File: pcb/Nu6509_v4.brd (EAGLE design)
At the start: 67.9 x 20.3 mm, 22 parts, among them IC1 6509, IC3 (C)02/'816, IC4 XC9572XL

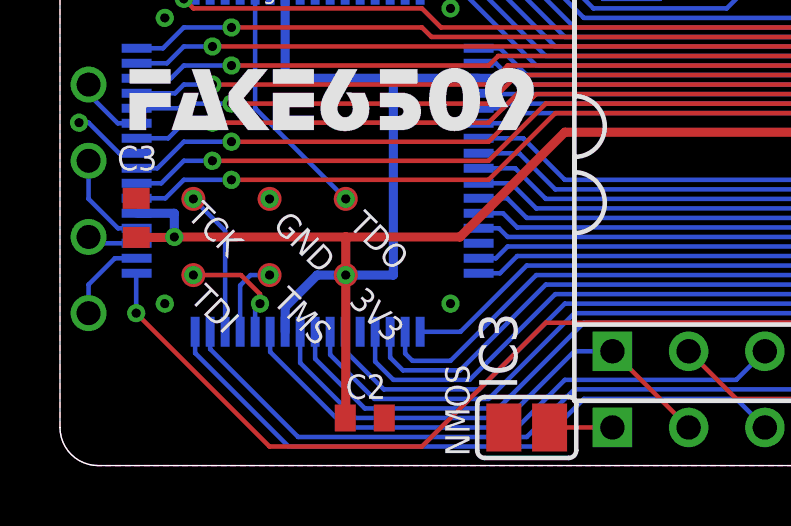
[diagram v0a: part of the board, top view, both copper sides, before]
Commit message: Switch name to Nu6509
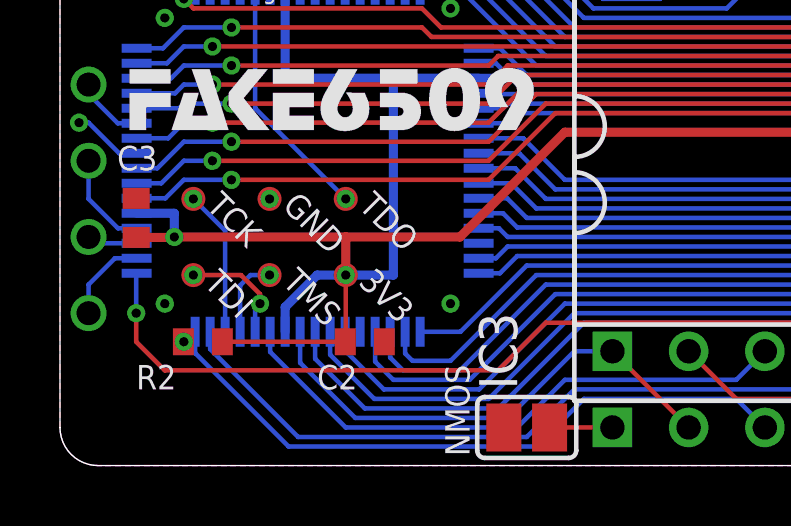
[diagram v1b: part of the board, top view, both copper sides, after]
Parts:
- added R2: 10K, rcl:R0402
- moved C2 2.54 mm to (-24.8, -6.03)
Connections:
- net !ABORT: now also R2.2
- net +3V3: now also R2.1
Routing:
- net +3V3: track 88.4 -> 90.0 mm
- net BE: track 96.6 -> 95.1 mm
- net !ABORT: track 22.0 -> 22.6 mm, vias 0 -> 1
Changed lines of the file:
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@@
 </autorouter>
 <elements>
-<element name="C2" library="rcl" package="C0402" value=".1" x="-24.765" y="-8.5725" smashed="yes">
-<attribute name="NAME" x="-25.4" y="-7.9375" size="0.8128" layer="25"/>
-<attribute name="VALUE" x="-27.305" y="-8.89" size="0.8128" layer="27"/>
+<element name="C2" library="rcl" package="C0402" value=".1" x="-24.765" y="-6.0325" smashed="yes">
+<attribute name="NAME" x="-26.3525" y="-7.62" size="0.8128" layer="25"/>
+<attribute name="VALUE" x="-24.13" y="-7.62" size="0.8128" layer="27"/>
 </element>
 <element name="C3" library="rcl" package="C0402" value=".1" x="-32.385" y="-1.905" smashed="yes" rot="R90">
 <attribute name="NAME" x="-33.02" y="-0.3175" size="0.8128" layer="25"/>
-<attribute name="VALUE" x="-32.7025" y="-4.445" size="0.8128" layer="27"/>
+<attribute name="VALUE" x="-32.7025" y="-4.445" size="0.8128" layer="27" ratio="10"/>
 </element>
 <element name="C4" library="rcl" package="C0402" value=".1" x="-28.2575" y="9.2075" smashed="yes" rot="R180">
@@
 <element name="TDI" library="testpad" package="TP08R" value="PTR1TP08R" x="-30.48" y="-3.81" smashed="yes">
 <attribute name="TP_SIGNAL_NAME" value="" x="-30.48" y="-5.715" size="1" layer="37"/>
-<attribute name="NAME" x="-30.633725" y="-4.623475" size="0.8128" layer="25" rot="R315"/>
+<attribute name="NAME" x="-30.1625" y="-4.1275" size="0.8128" layer="25" ratio="10" rot="R315"/>
 </element>
 <element name="TMS" library="testpad" package="TP08R" value="PTR1TP08R" x="-27.94" y="-3.81" smashed="yes">
 <attribute name="TP_SIGNAL_NAME" value="" x="-27.94" y="-5.715" size="1" layer="37"/>
-<attribute name="NAME" x="-27.869215625" y="-4.71646875" size="0.8128" layer="25" rot="R315"/>
+<attribute name="NAME" x="-27.551715625" y="-4.08146875" size="0.8128" layer="25" rot="R315"/>
 </element>
 <element name="TCK" library="testpad" package="TP08R" value="PTR1TP08R" x="-30.48" y="-1.27" smashed="yes">
 <attribute name="TP_SIGNAL_NAME" value="" x="-30.48" y="-3.175" size="1" layer="37"/>
-<attribute name="NAME" x="-30.726715625" y="-1.85896875" size="0.8128" layer="25" rot="R315"/>
+<attribute name="NAME" x="-30.091715625" y="-1.54146875" size="0.8128" layer="25" rot="R315"/>
 </element>
 <element name="3V3" library="testpad" package="TP08R" value="PTR1TP08R" x="-25.4" y="-3.81" smashed="yes">
 <attribute name="TP_SIGNAL_NAME" value="" x="-25.4" y="-5.715" size="1" layer="37"/>
-<attribute name="NAME" x="-25.329215625" y="-4.71646875" size="0.8128" layer="25" rot="R315"/>
+<attribute name="NAME" x="-25.011715625" y="-4.08146875" size="0.8128" layer="25" rot="R315"/>
 </element>
 <element name="TDO" library="testpad" package="TP08R" value="PTR1TP08R" x="-25.4" y="-1.27" smashed="yes">
 <attribute name="TP_SIGNAL_NAME" value="" x="-25.4" y="-3.175" size="1" layer="37"/>
-<attribute name="NAME" x="-25.329215625" y="-2.17646875" size="0.8128" layer="25" rot="R315"/>
+<attribute name="NAME" x="-25.011715625" y="-1.54146875" size="0.8128" layer="25" rot="R315"/>
 </element>
 <element name="GND" library="testpad" package="TP08R" value="PTR1TP08R" x="-27.94" y="-1.27" smashed="yes">
 <attribute name="TP_SIGNAL_NAME" value="" x="-27.94" y="-3.175" size="1" layer="37"/>
-<attribute name="NAME" x="-27.869215625" y="-2.17646875" size="0.8128" layer="25" rot="R315"/>
+<attribute name="NAME" x="-27.551715625" y="-1.54146875" size="0.8128" layer="25" rot="R315"/>
 </element>
 <element name="PORT4" library="testpad" package="TP08R" value="PTR1TP08R" x="-33.9725" y="2.54" smashed="yes" rot="MR0">
@@
 <attribute name="NAME" x="-22.5425" y="8.89" size="0.8128" layer="25"/>
 <attribute name="VALUE" x="-20.6375" y="8.89" size="0.8128" layer="27"/>
+</element>
+<element name="R2" library="rcl" package="R0402" value="10K" x="-30.1625" y="-6.0325" smashed="yes" rot="R180">
+<attribute name="NAME" x="-32.385" y="-7.62" size="0.8128" layer="25" ratio="10"/>
+<attribute name="VALUE" x="-30.48" y="-7.62" size="0.8128" layer="27" ratio="10"/>
 </element>
 </elements>
@@
 <wire x1="-27.42" y1="-4.8775" x2="-26.3525" y2="-3.81" width="0.3048" layer="16"/>
 <wire x1="-26.3525" y1="-3.81" x2="-25.4" y2="-3.81" width="0.3048" layer="16"/>
-<wire x1="-25.415" y1="-8.5725" x2="-25.4" y2="-8.5725" width="0.3048" layer="1"/>
-<wire x1="-25.4" y1="-8.5725" x2="-25.4" y2="-3.81" width="0.3048" layer="1"/>
+<wire x1="-25.415" y1="-6.0325" x2="-25.4" y2="-6.0325" width="0.1524" layer="1"/>
+<wire x1="-25.4" y1="-6.0325" x2="-25.4" y2="-3.81" width="0.1524" layer="1"/>
 <wire x1="-27.42" y1="5.7" x2="-27.42" y2="6.6675" width="0.3048" layer="16"/>
 <wire x1="-27.42" y1="6.6675" x2="-27.6225" y2="6.6675" width="0.3048" layer="16"/>
@@
 <wire x1="9.525" y1="0" x2="8.5725" y2="0.9525" width="0.3048" layer="1"/>
 <wire x1="8.5725" y1="0.9525" x2="-18.0975" y2="0.9525" width="0.3048" layer="1"/>
+<contactref element="R2" pad="1"/>
+<wire x1="-29.5125" y1="-6.0325" x2="-25.415" y2="-6.0325" width="0.1524" layer="1"/>
 </signal>
 <signal name="!ABORT">
@@
 <wire x1="-17.4625" y1="-7.9375" x2="-12.3825" y2="-7.9375" width="0.1524" layer="16"/>
 <wire x1="-12.3825" y1="-7.9375" x2="-11.43" y2="-8.89" width="0.1524" layer="16"/>
+<contactref element="R2" pad="2"/>
+<wire x1="-30.8125" y1="-6.0325" x2="-30.7975" y2="-6.0325" width="0.1524" layer="1"/>
+<via x="-30.7975" y="-6.0325" extent="1-16" drill="0.3048"/>
+<wire x1="-30.7975" y1="-6.0325" x2="-30.42" y2="-6.41" width="0.1524" layer="16"/>
 </signal>
 <signal name="!RDY">
@@
 <wire x1="-6.35" y1="-6.35" x2="-7.3025" y2="-5.3975" width="0.1524" layer="1"/>
 <wire x1="-7.3025" y1="-5.3975" x2="-18.7325" y2="-5.3975" width="0.1524" layer="1"/>
-<wire x1="-18.7325" y1="-5.3975" x2="-22.86" y2="-9.525" width="0.1524" layer="1"/>
-<wire x1="-22.86" y1="-9.525" x2="-27.94" y2="-9.525" width="0.1524" layer="1"/>
-<wire x1="-27.94" y1="-9.525" x2="-32.385" y2="-5.08" width="0.1524" layer="1"/>
+<wire x1="-18.7325" y1="-5.3975" x2="-20.32" y2="-6.985" width="0.1524" layer="1"/>
+<wire x1="-20.32" y1="-6.985" x2="-31.4325" y2="-6.985" width="0.1524" layer="1"/>
+<wire x1="-31.4325" y1="-6.985" x2="-32.385" y2="-6.0325" width="0.1524" layer="1"/>
+<wire x1="-32.385" y1="-6.0325" x2="-32.385" y2="-5.08" width="0.1524" layer="1"/>
 <via x="-32.385" y="-5.08" extent="1-16" drill="0.3048"/>
 <wire x1="-32.385" y1="-5.08" x2="-32.385" y2="-3.765" width="0.1524" layer="16"/>

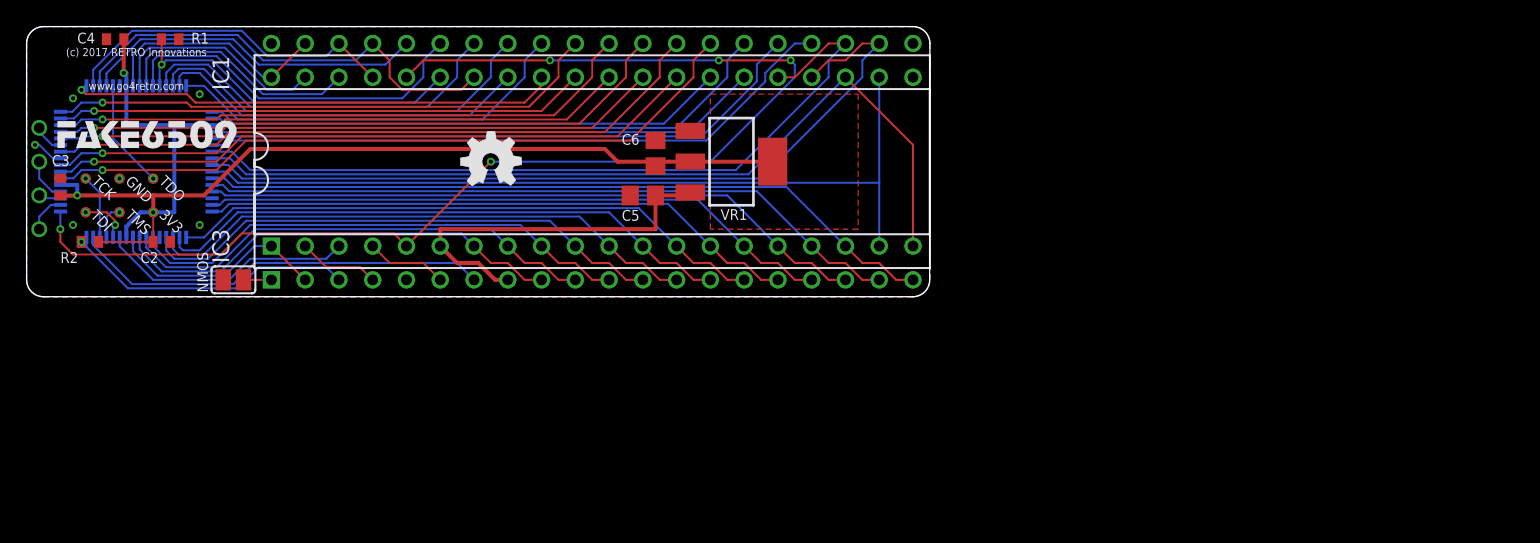
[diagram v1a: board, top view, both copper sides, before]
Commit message: Added JED file
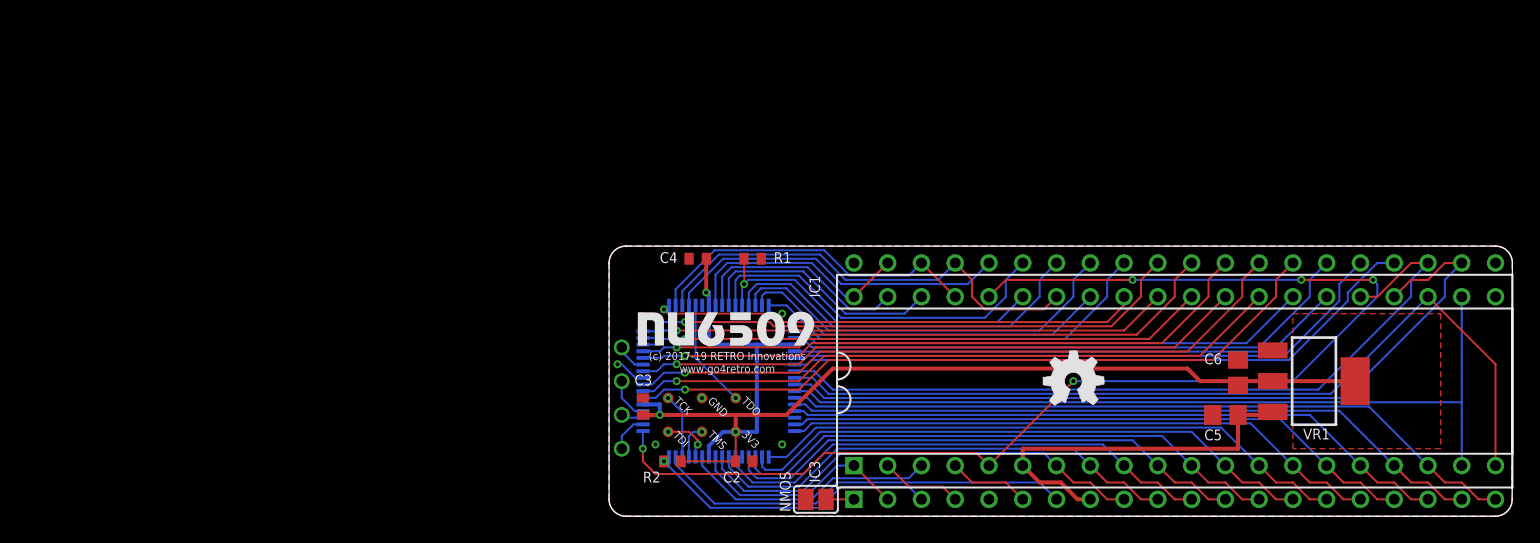
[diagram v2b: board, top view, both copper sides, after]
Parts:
- moved IC1 46.8 mm to (51.4, -15.2)
- moved IC3 46.8 mm to (51.4, -17.8)
- moved 3V3 46.8 mm to (18.4, -20.3)
- moved C2 46.8 mm to (19.1, -22.5)
- moved C3 46.8 mm to (11.4, -18.4)
- moved C4 46.8 mm to (15.6, -7.30)
- moved C5 46.8 mm to (55.2, -19.1)
- moved C6 46.8 mm to (56.2, -15.9)
- moved GND 46.8 mm to (15.9, -17.8)
- moved GOLD_ORB_SM1 46.8 mm to (43.8, -16.5)
- moved IC4 46.8 mm to (17.1, -16.5)
- moved NMOS 46.8 mm to (24.4, -25.4)
- moved PORT4 46.8 mm to (9.84, -14.0)
- moved PORT5 46.8 mm to (9.84, -16.5)
- moved PORT6 46.8 mm to (9.84, -19.1)
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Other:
- outline, holes or cut-outs redrawn
- board text added: "(c) 2017-19 RETRO Innovations"
- board text added: "C:/Users/brain/projects/Nu6509/doc/Nu6509.bmp"
- board text removed: "(c) 2017 RETRO Innovations"
